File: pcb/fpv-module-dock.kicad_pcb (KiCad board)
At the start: 2 copper layers, 80 x 50 mm, 12 parts, among them J1 Barrel_Jack_Switch, J2 AudioJack4_SwitchTR1, J3 Conn_01x09, SW1 SW_SPDT, SW2 SW_Push, SW3 SW_Push, SW4 SW_Push, U1 2850

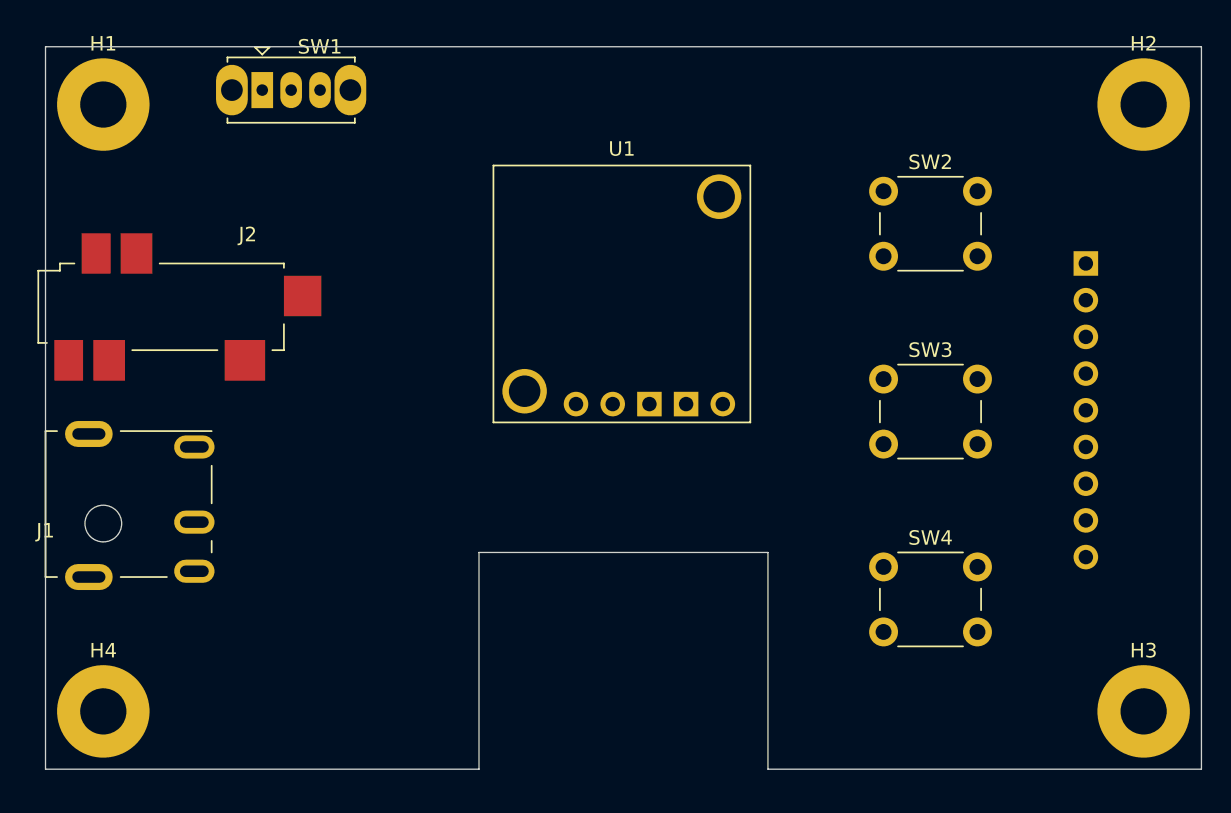
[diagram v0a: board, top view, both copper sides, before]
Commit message: Working on layout
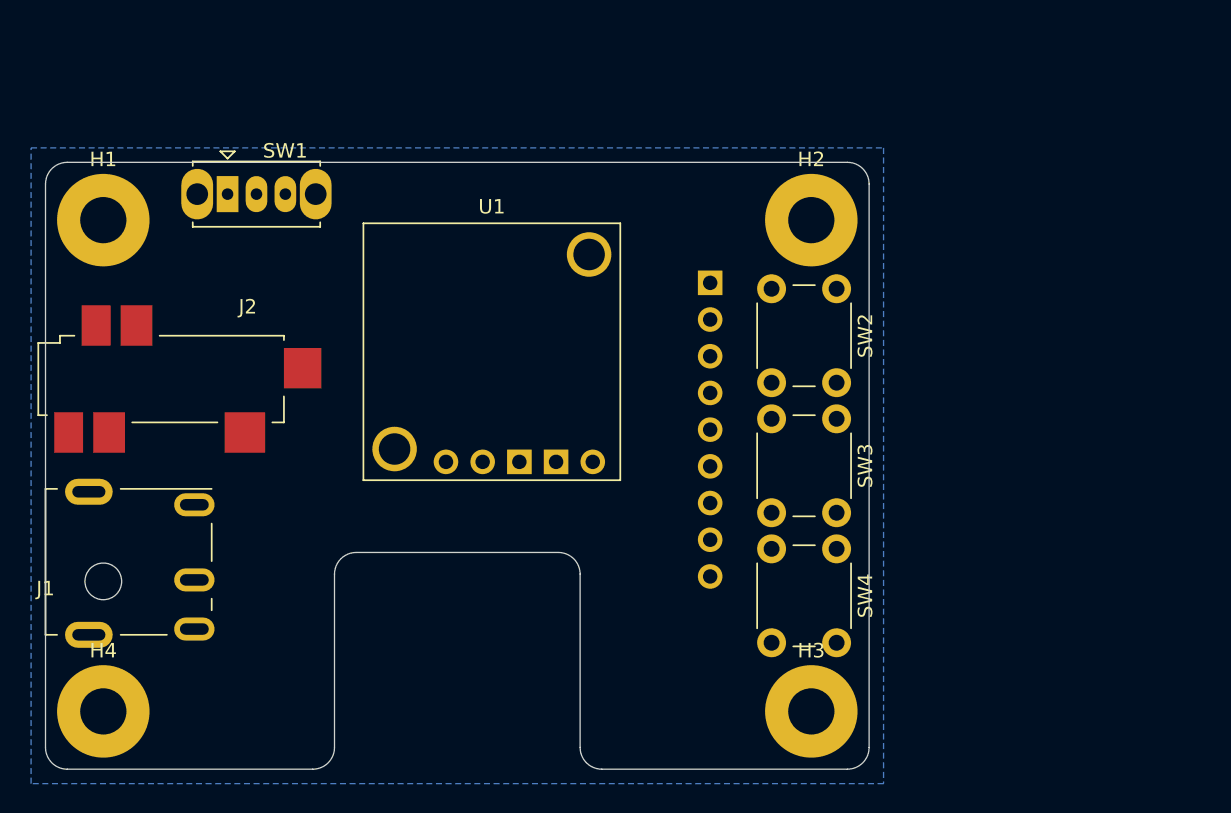
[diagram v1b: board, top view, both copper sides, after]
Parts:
- moved J3 26.0 mm to (156.0, 91.3)
- moved H2 24.4 mm to (163.0, 87.0)
- moved H3 23.0 mm to (163.0, 121.0)
- moved U1 9.85 mm to (132.0, 105.0)
- moved H1 8.00 mm to (114.0, 87.0)
- moved SW1 7.59 mm to (122.6, 85.2)
- moved SW2 7.49 mm to (164.8, 91.8), turned to 270 degrees
- moved J2 5.00 mm to (111.0, 98.0)
- moved SW3 4.26 mm to (164.8, 100.8), turned to 270 degrees
- moved J1 4.00 mm to (110.0, 112.0)
- moved SW4 3.48 mm to (164.8, 109.8), turned to 270 degrees
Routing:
- added copper zone on B.Cu, net GND
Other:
- board size 80 x 50 mm -> 57 x 42 mm

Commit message: Added 3D models, completed layout
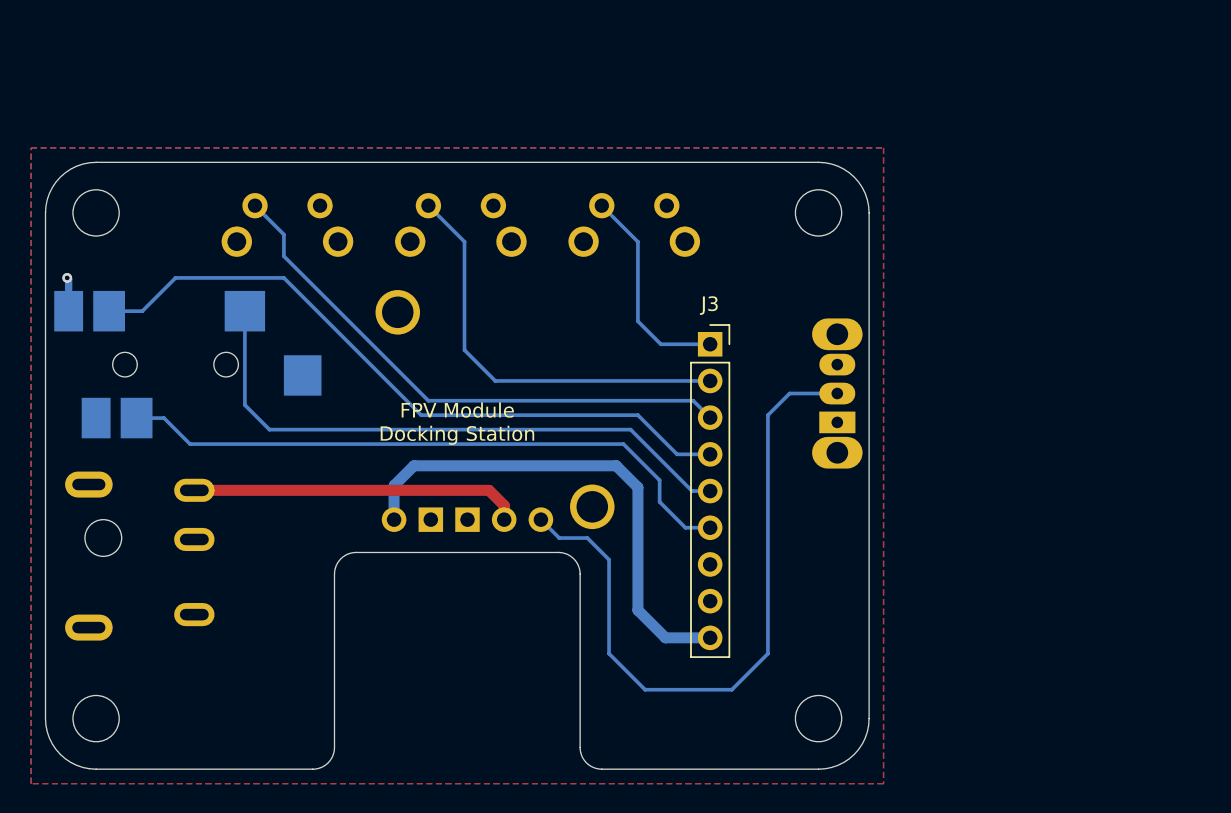
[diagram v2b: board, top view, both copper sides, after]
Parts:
- H1, H2, H3, H4: footprint MountingHole:MountingHole_3.2mm_M3_Pad -> MountingHole:MountingHole_3.2mm_M3
- J1, J2, U1: moved to B.Cu
- J3: moved to F.Cu
- SW1: footprint Button_Switch_THT:SW_Slide_1P2T_CK_OS102011MS2Q -> fpv-module-dock:OS102011MA1QN1; moved to B.Cu
- SW2, SW3, SW4: footprint Button_Switch_THT:SW_PUSH_6mm_H13mm -> Button_Switch_THT:SW_Tactile_SPST_Angled_PTS645Vx83-2LFS; moved to B.Cu
- moved SW1 45.1 mm to (164.8, 101.0), turned to 90 degrees
- moved SW4 42.9 mm to (129.0, 86.0), turned to 180 degrees
- moved SW3 28.0 mm to (141.0, 86.0), turned to 180 degrees
- moved U1 18.4 mm to (150.0, 109.0), turned to 180 degrees
- moved SW2 13.1 mm to (153.0, 86.0), turned to 180 degrees
- moved J3 4.25 mm to (156.0, 95.6), turned to 0 degrees
- moved J1 3.00 mm to (110.0, 109.0)
- moved J2 1.00 mm to (111.0, 97.0)
- moved H1 0.71 mm to (113.5, 86.5)
- moved H2 0.71 mm to (163.5, 86.5)
- moved H3 0.71 mm to (163.5, 121.5)
- moved H4 0.71 mm to (113.5, 121.5)
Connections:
- SW1 pad 1: Net-(SW1-Pad1) -> GND
- SW1 pad 3: GND -> Net-(SW1-Pad3)
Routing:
- net /VIDEO: track 0.00 -> 47.6 mm
- net Net-(SW1-Pad2): track 0.00 -> 47.4 mm
- net /AUDIO_R: track 0.00 -> 43.7 mm
- net /AUDIO_L: track 0.00 -> 41.2 mm
- net Net-(J3-Pad3): track 0.00 -> 38.5 mm
- net +5V: track 0.00 -> 34.7 mm
- net Net-(J3-Pad2): track 0.00 -> 28.9 mm
- net +BATT: track 0.00 -> 22.9 mm
- net Net-(J3-Pad1): track 0.00 -> 14.7 mm
- net GND: track 0.00 -> 2.34 mm, vias 0 -> 1
- added copper zone on B.Cu, net (none)
- added copper zone on F.Cu, net GND
- removed copper zone on B.Cu, net GND
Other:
- outline, holes or cut-outs redrawn
- net class Default: clearance 0.2 -> 0.1524; trace_width 0.25 -> 0.1524; via_dia 0.8 -> 0.6858; via_drill 0.4 -> 0.3302
- net class Power added: clearance 0.1524, trace_width 0.762, via_dia 0.6858, via_drill 0.3302
- rule pad_to_mask_clearance: 0 -> 0.000051
- rule trace_clearance: 0.2 -> 0.1524
- rule trace_min: 0.2 -> 0.1524
- rule via_min_drill: 0.3 -> 0.254
- rule via_min_size: 0.4 -> 0.508
- board text added: "FPV Module Docking Station"
